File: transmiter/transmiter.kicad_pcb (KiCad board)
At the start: 2 copper layers, 54.4 x 48.3 mm, 64 parts, among them J1 USB_B_Mini, J2 Conn_01x04_Pin, J3 Conn_01x04_Pin, SW1 SW_Push, SW2 SW_SPDT, U1 ADL5370, U2 STM32F303K8Tx, U3 AMS1117-3.3, U4 ADL5531, U5 Si590, U6 FIN1001M5X, U7 FIN1001M5X, U9 FT232RL, Y1 16MHz

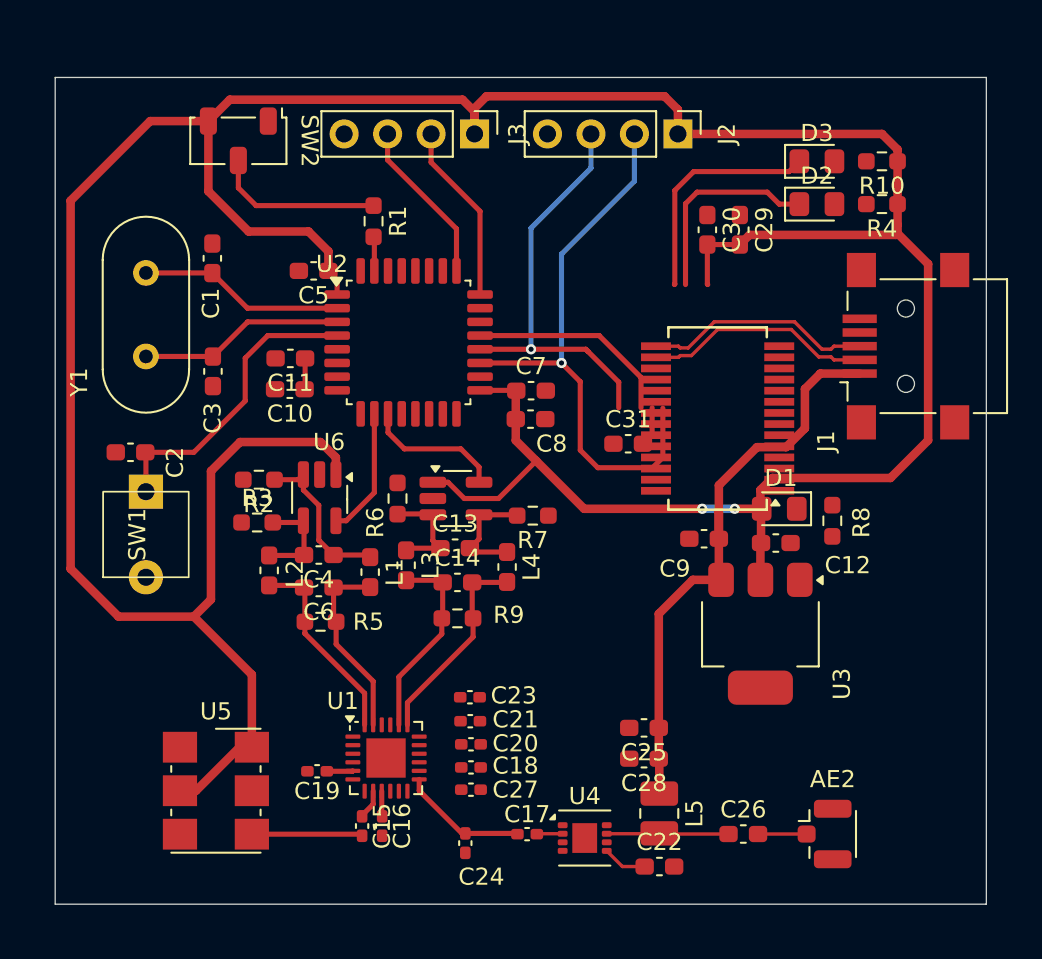
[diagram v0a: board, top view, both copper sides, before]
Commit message: Finished PCB design
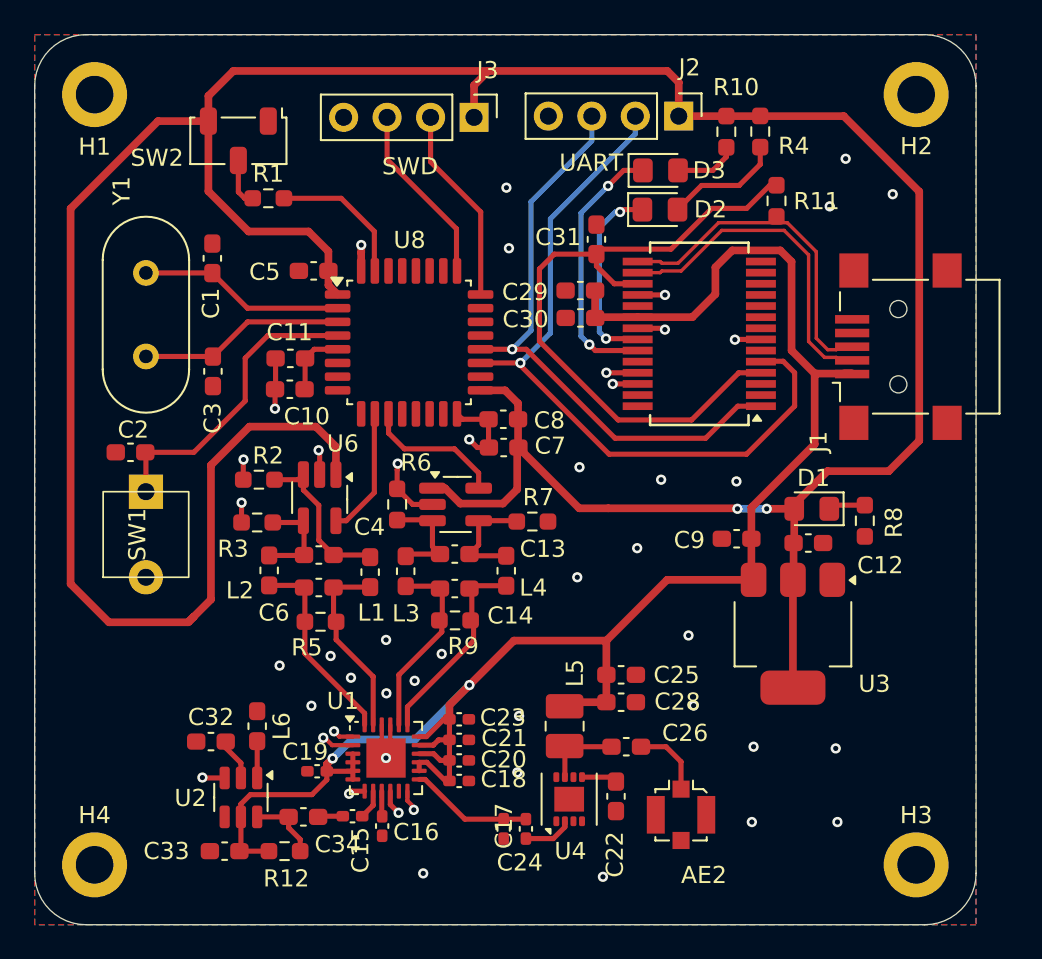
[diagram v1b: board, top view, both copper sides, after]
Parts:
- removed C27: C, Capacitor_SMD:C_0402_1005Metric_Pad0.74x0.62mm_HandSolder
- removed U5: Si590, Oscillator:Oscillator_SMD_IDT_JU6-6_7.0x5.0mm_P2.54mm
- added C32: C, Capacitor_SMD:C_0603_1608Metric_Pad1.08x0.95mm_HandSolder, F.Cu at (92.3, 92.3)
- added C33: C, Capacitor_SMD:C_0603_1608Metric_Pad1.08x0.95mm_HandSolder, F.Cu at (93.1, 98.7)
- added C34: C, Capacitor_SMD:C_0603_1608Metric_Pad1.08x0.95mm_HandSolder, F.Cu at (97.7, 96.7)
- added H1: MountingHole_Pad, MountingHole:MountingHole_2.2mm_M2_DIN965_Pad, F.Cu at (85.5, 54.5)
- added H2: MountingHole_Pad, MountingHole:MountingHole_2.2mm_M2_DIN965_Pad, F.Cu at (133.5, 54.5)
- added H3: MountingHole_Pad, MountingHole:MountingHole_2.2mm_M2_DIN965_Pad, F.Cu at (133.5, 99.5)
- added H4: MountingHole_Pad, MountingHole:MountingHole_2.2mm_M2_DIN965_Pad, F.Cu at (85.5, 99.5)
- added L6: 18n, Inductor_SMD:L_0603_1608Metric_Pad1.05x0.95mm_HandSolder, F.Cu at (95.0, 91.4)
- added R11: 1.5k, Resistor_SMD:R_0603_1608Metric_Pad0.98x0.95mm_HandSolder, F.Cu at (125.3, 60.7)
- added R12: 1k, Resistor_SMD:R_0603_1608Metric_Pad0.98x0.95mm_HandSolder, F.Cu at (96.6, 98.7)
- added U8: STM32F303K8Tx, Package_QFP:LQFP-32_7x7mm_P0.8mm, F.Cu at (103.9, 69.0)
- AE2: footprint Connector_Coaxial:U.FL_Hirose_U.FL-R-SMT-1_Vertical -> Connector_Coaxial:U.FL_Molex_MCRF_73412-0110_Vertical
- U2: value STM32F303K8Tx -> MAX2608; footprint Package_QFP:LQFP-32_7x7mm_P0.8mm -> Package_TO_SOT_SMD:SOT-23-6
- moved U2 28.3 mm to (94.0, 95.6), turned to -90 degrees
- moved C31 12.1 mm to (114.8, 63.0), turned to -90 degrees
- moved C29 9.97 mm to (113.9, 66.0), turned to 0 degrees
- moved R10 9.25 mm to (122.4, 56.7), turned to -90 degrees
- moved D2 9.17 mm to (118.5, 61.2)
- moved D3 9.16 mm to (118.6, 58.9)
- moved C30 9.03 mm to (113.9, 67.5), turned to 0 degrees
- moved C26 8.53 mm to (116.6, 92.6)
- moved AE2 8.46 mm to (119.8, 96.6), turned to 180 degrees
- moved R4 8.28 mm to (124.4, 56.7), turned to -90 degrees
- moved L5 7.52 mm to (113.0, 91.4)
- moved R1 6.29 mm to (95.7, 60.6), turned to 0 degrees
- moved U9 5.06 mm to (120.8, 68.5)
- moved C22 4.82 mm to (116.0, 95.5), turned to -90 degrees
- moved C7 3.69 mm to (109.4, 75.1), turned to 180 degrees
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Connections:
- net Net-(U9-3V3OUT) renamed 3V3
- C29 pad 2: +3V3 -> +5V
- C30 pad 2: +3V3 -> +5V
- U2 pad 1: +3V3 -> Net-(U2-IND)
- U2 pad 2: HSE_IN -> Net-(U2-TUNE)
- U2 pad 3: HSE_OUT -> GND
- U2 pad 4: NRST -> unconnected-(U2-OUT--Pad4)
- U2 pad 5: +3VA3 -> +5V
- U2 pad 6: unconnected-(U2-PA0-Pad6) -> Net-(U2-OUT+)
- U9 pad 11: USART1_RTS -> unconnected-(U9-CTS-Pad11)
- U9 pad 20: +3V3 -> +5V
- U9 pad 26: unconnected-(U9-TEST-Pad26) -> GND
- U9 pad 3: USART1_CTS -> unconnected-(U9-RTS-Pad3)
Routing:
- net +5V: track 36.1 -> 103.8 mm, vias 0 -> 2
- net 3V3: track 2.32 -> 39.6 mm
- net GND: track 0.00 -> 37.1 mm, vias 0 -> 47
- net +3V3: track 210.2 -> 191.9 mm
- net USART1_CTS: track 12.2 -> 0.00 mm
- net USART1_RX: track 24.6 -> 34.9 mm
- net USART1_TX: track 33.8 -> 43.2 mm
- net Net-(SW2-B): track 9.93 -> 2.83 mm
- net Net-(D2-A): track 0.00 -> 6.94 mm
- net BOOT: track 2.01 -> 8.39 mm
- net USB_D+: track 13.3 -> 19.7 mm
- net USB_D-: track 13.3 -> 19.7 mm
- net LOIP: track 6.48 -> 1.46 mm
- net Net-(U2-OUT+): track 0.00 -> 4.12 mm
- net Net-(D3-A): track 0.00 -> 3.71 mm
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- added copper zone on B.Cu, net GND
- added copper zone on F.Cu, net GND
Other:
- board size 54.4 x 48.3 mm -> 55 x 52 mm
- board text added: "SWD"
- board text added: "UART"
